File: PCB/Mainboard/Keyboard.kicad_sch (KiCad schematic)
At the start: 36 parts, among them J16 Keyboard Conn 2, J17 Keyboard Conn 1, J19 Trackpoint, Q8 MUN2114, U69 SN74LVC2G32, U73 SN74LVT244B, X5 4.00, X6 8.00

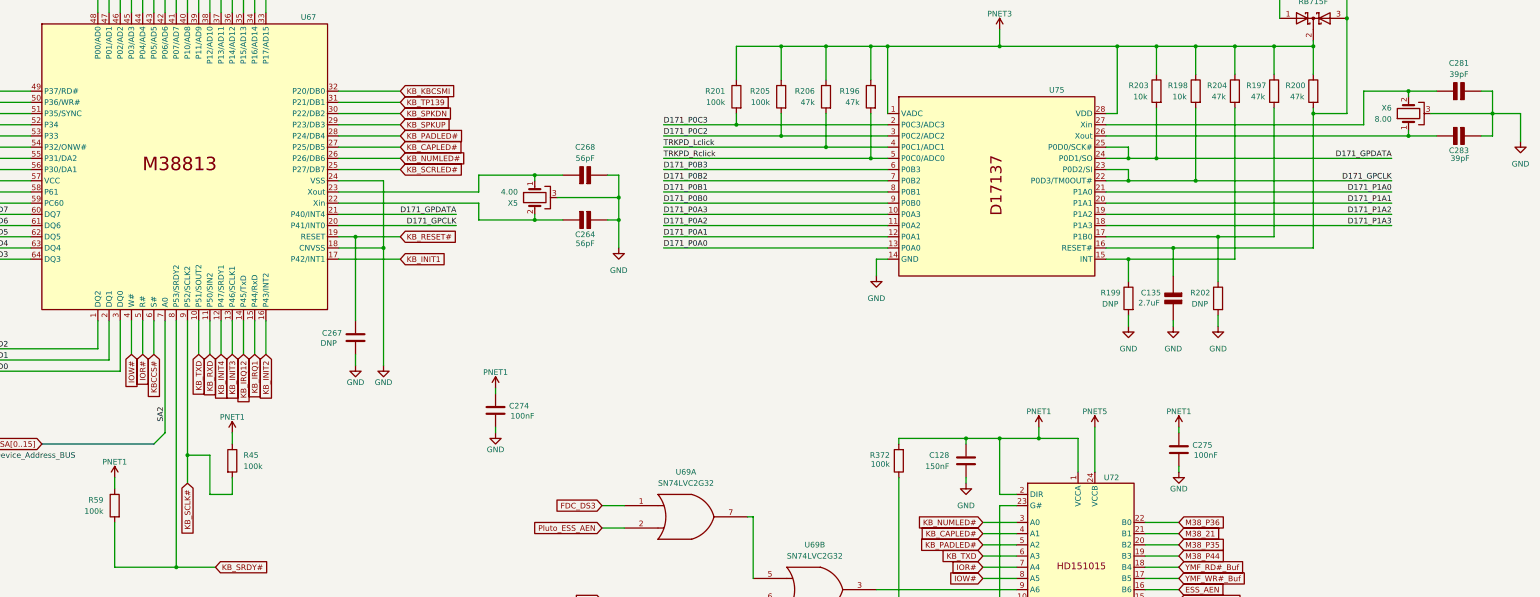
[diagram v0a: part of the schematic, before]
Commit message: Add files via upload
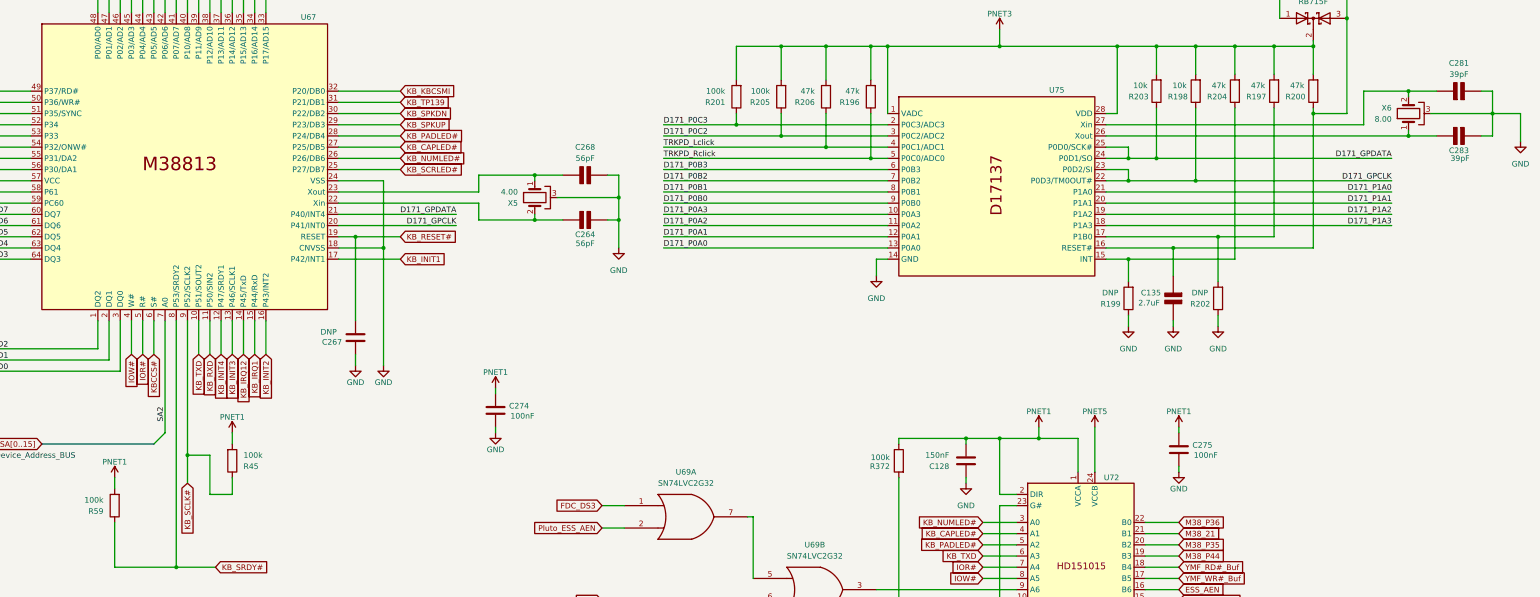
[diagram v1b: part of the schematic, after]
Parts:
- C128, C136, C264, C267, C268, C274, C275, C281, C283: footprint (none) -> Capacitor_SMD:C_0402_1005Metric
- C135: footprint (none) -> Capacitor_SMD:C_0805_2012Metric
- D35, Q8: footprint (none) -> PC110:3D
- J16: footprint (none) -> PC110:Flat-20
- J17: footprint (none) -> PC110:Flat-8
- J19: footprint (none) -> PC110:Flat-18
- R196, R197, R198, R199, R200, R201, R202, R203, R204, R205, R206, R45, R59: footprint (none) -> PCM_Resistor_SMD_AKL:R_0402_1005Metric
- R372: footprint (none) -> Resistor_SMD:R_0402_1005Metric
- U67: footprint (none) -> PC110:QFN64
- U69: footprint (none) -> Package_SO:SSOP-8_2.95x2.8mm_P0.65mm
- U72: footprint (none) -> Package_SO:SSOP-24_5.3x8.2mm_P0.65mm
- U73: footprint (none) -> Package_SO:TSSOP-20_4.4x6.5mm_P0.65mm
- U75: footprint (none) -> PC110:SSOP-28
- X5: footprint (none) -> PC110:XTAL-5
- X6: footprint (none) -> PC110:XTAL-4
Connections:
- net Bowman_ESS_DACK1#: now also R372.2; no longer R372.1
- net D171_GPCLK: now also R198.1; no longer R198.2
- net D171_GPDATA: now also R203.1; no longer R203.2
- net D171_P0C2: now also R205.1; no longer R205.2
- net D171_P0C3: now also R201.1; no longer R201.2
- net GND: now also C128.2, C264.1 (+), C267.1, C268.1 (+), C281.1 (+), R199.1, R202.1; no longer C128.1, C264.2 (-), C267.2, C268.2 (-), C281.2 (-), R199.2, R202.2
- net KB_RESET#: now also C267.2; no longer C267.1
- net KB_SCLK#: now also R45.1; no longer R45.2
- net KB_SRDY#: now also R59.1; no longer R59.2
- net PNET1: now also C128.1, R372.1, R45.2, R59.2; no longer C128.2, R372.2, R45.1, R59.1
- net PNET3: now also R196.2, R197.2, R198.2, R200.2, R201.2, R203.2, R204.2, R205.2, R206.2; no longer R196.1, R197.1, R198.1, R200.1, R201.1, R203.1, R204.1, R205.1, R206.1
- net TRKPD_Lclick: now also R206.1; no longer R206.2
- net TRKPD_Rclick: now also R196.1; no longer R196.2
- net at C135.1 (+), D35.1 (A), D35.3 (A)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: now also R200.1; no longer R200.2
- net at U75.27 (Xin), X6.2: now also C281.2 (-); no longer C281.1 (+)
- net at U67.22 (Xin), X5.2: now also C264.2 (-); no longer C264.1 (+)
- net at U67.23 (Xout), X5.1: now also C268.2 (-); no longer C268.1 (+)
- new net: R197.1, R202.2, U75.17 (P1B0)
- new net: R199.2, R204.1, U75.15 (INT)
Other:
- moved on the sheet: C264, C268, C281, R196, R197, R198, R199, R200, R201, R202, R203, R204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
